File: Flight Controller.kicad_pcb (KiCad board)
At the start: 4 copper layers, 39.5 x 39.5 mm, 136 parts, among them IC2 AT7456E, J1 Conn_01x08_MountingPin, J2 USB_C_Receptacle_USB2.0_14P, Q2 BC817W, U1 AT32F435RGT7, U2 LMR51430, U3 BMP280, U4 NCP1117-3.3_SOT223, U5 LMR51430, U6 W25Q128JVSIQ TR, U7 ICM-42688-P, U8 NCP1117-3.3_SOT223, Y1 8M, Y2 27M

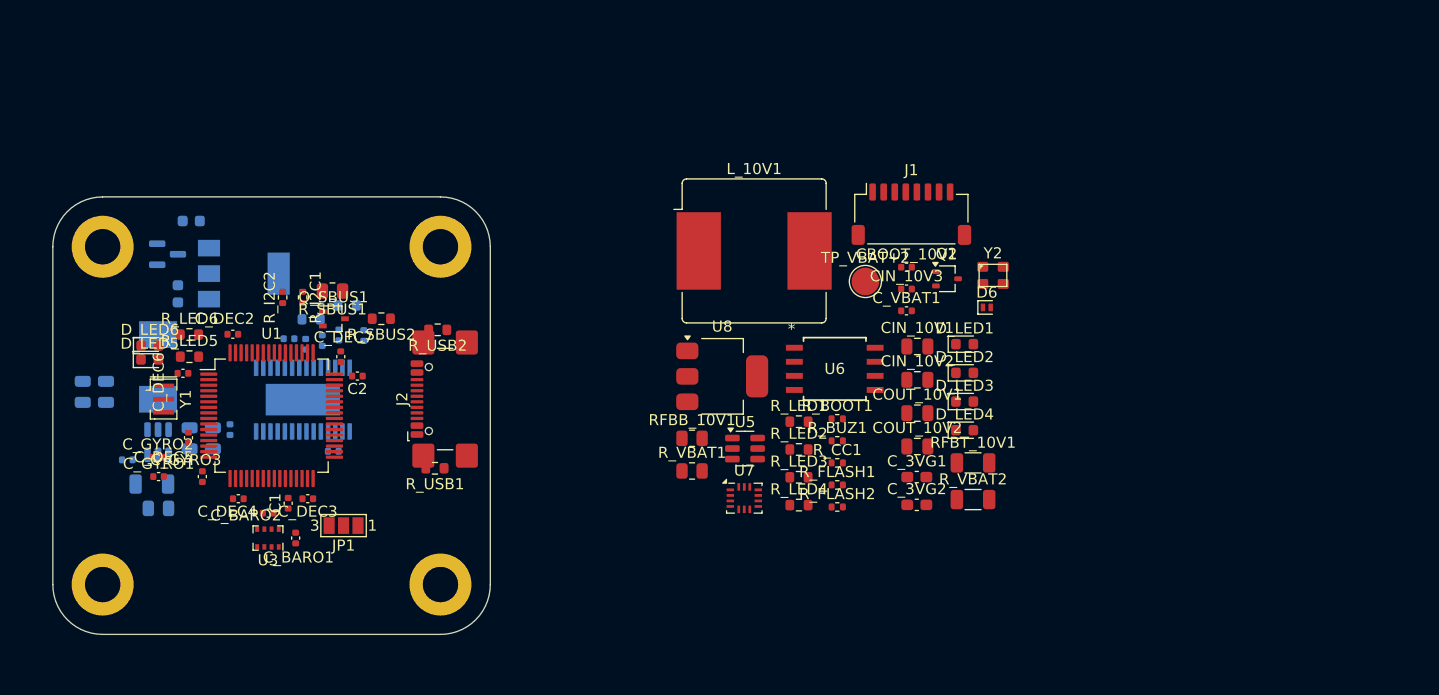
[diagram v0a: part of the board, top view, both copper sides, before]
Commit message: First Layout
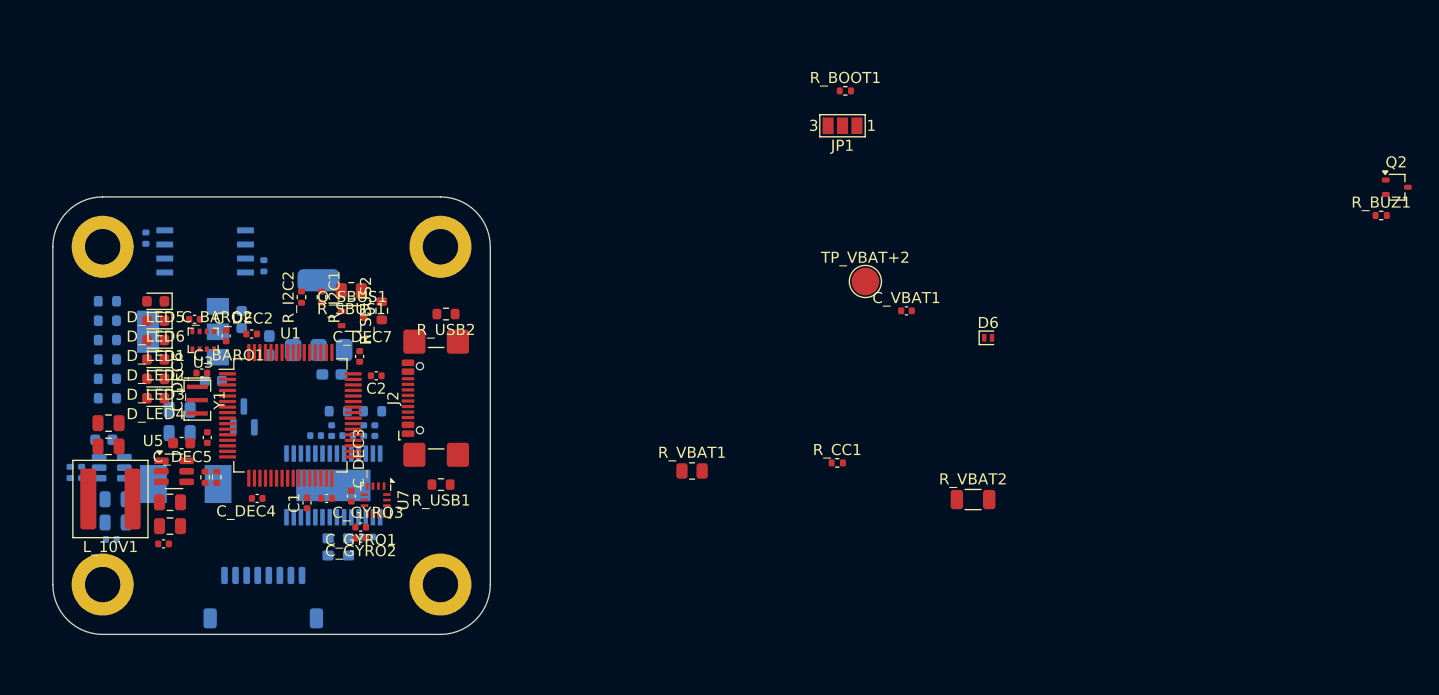
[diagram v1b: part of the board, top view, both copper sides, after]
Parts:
- CBOOT_10V1, CBOOT_5V1: footprint Capacitor_SMD:C_0402_1005Metric -> Capacitor_SMD:C_0603_1608Metric
- C_3VG1, C_3VG2, J1, R_FLASH1, R_FLASH2, R_LED1, R_LED2, R_LED3, R_LED4, R_LED5, R_LED6, U6, U8, Y2: moved to B.Cu
- L_10V1: footprint Inductor_SMD:L_Bourns_SRR1208_12.7x12.7mm -> Wurth-Elektronik:744393465120
- RFBB_10V1, RFBB_5V1: footprint Resistor_SMD:R_0805_2012Metric -> Resistor_SMD:R_0402_1005Metric
- RFBT_10V1, RFBT_5V1: footprint Resistor_SMD:R_1206_3216Metric -> Resistor_SMD:R_0402_1005Metric
- moved D_LED4 73.1 mm to (134.5, 83.5), turned to 180 degrees
- moved D_LED3 73.1 mm to (134.5, 81.8), turned to 180 degrees
- moved D_LED2 73.1 mm to (134.5, 80.0), turned to 180 degrees
- moved D_LED1 73.0 mm to (134.5, 78.2), turned to 180 degrees
- moved COUT_10V1 73.0 mm to (130.3, 85.8)
- moved COUT_10V2 73.0 mm to (130.3, 87.8)
- moved CIN_10V3 70.9 mm to (135.2, 96.7), turned to 180 degrees
- moved RFBT_10V1 69.3 mm to (139.0, 90.6), turned to -90 degrees
- moved CIN_10V1 68.9 mm to (135.8, 92.9)
- moved CIN_10V2 68.8 mm to (135.8, 95.0)
- moved J1 68.0 mm to (144.2, 101.5), turned to 180 degrees
- moved CBOOT_10V1 67.3 mm to (136.9, 87.5), turned to 180 degrees
- moved R_FLASH1 66.3 mm to (133.7, 69.0), turned to -90 degrees
- moved Y2 64.0 mm to (151.0, 96.9), turned to 180 degrees
- moved R_LED4 63.2 mm to (130.2, 83.5)
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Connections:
- D2 pad 1: +5V -> /5V_USB
- D2 pad 2: /5V_USB -> +5V
